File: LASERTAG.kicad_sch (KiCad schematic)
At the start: 38 parts, among them J1 Conn_01x02_Pin, J2 USB_C_Receptacle_USB2.0_14P, J3 Conn_01x02_Pin, SW1 SW_Push, SW2 SW_Push, SW3 SW_SPST, SW4 SW_SPST, U1 ATMEGA328-AU, U2 ESP32-S2-SOLO, U3 TPS613221ADBVR, U4 TPS613221ADBVR, U5 AP7366-33W5-7, U6 TSOP582xx, U7 TLV61048DBVR

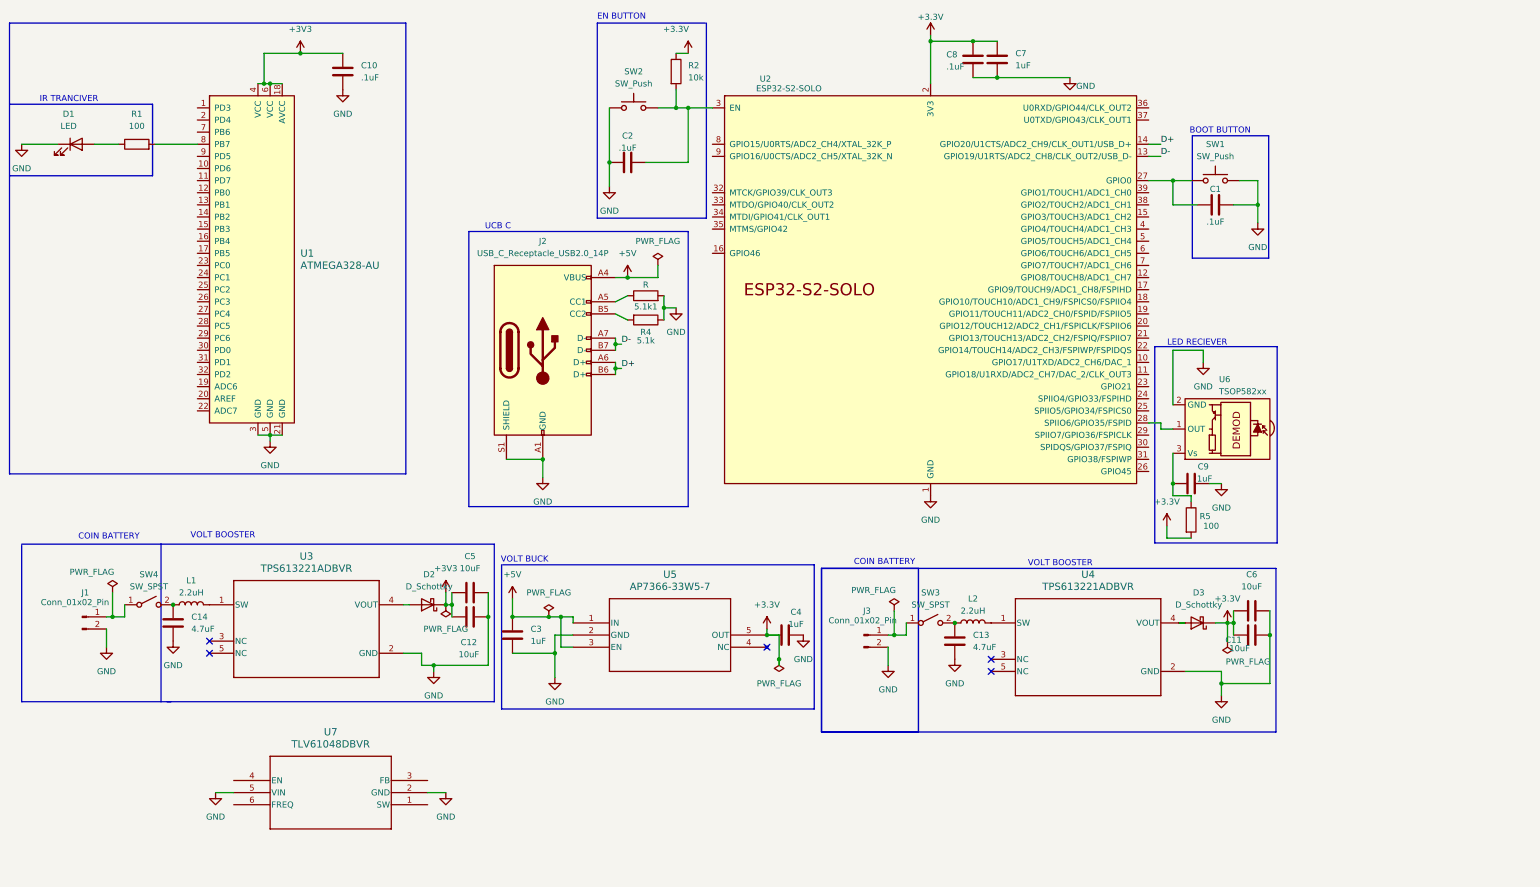
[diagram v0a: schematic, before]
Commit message: fix a lot of things i don't remember sorryy
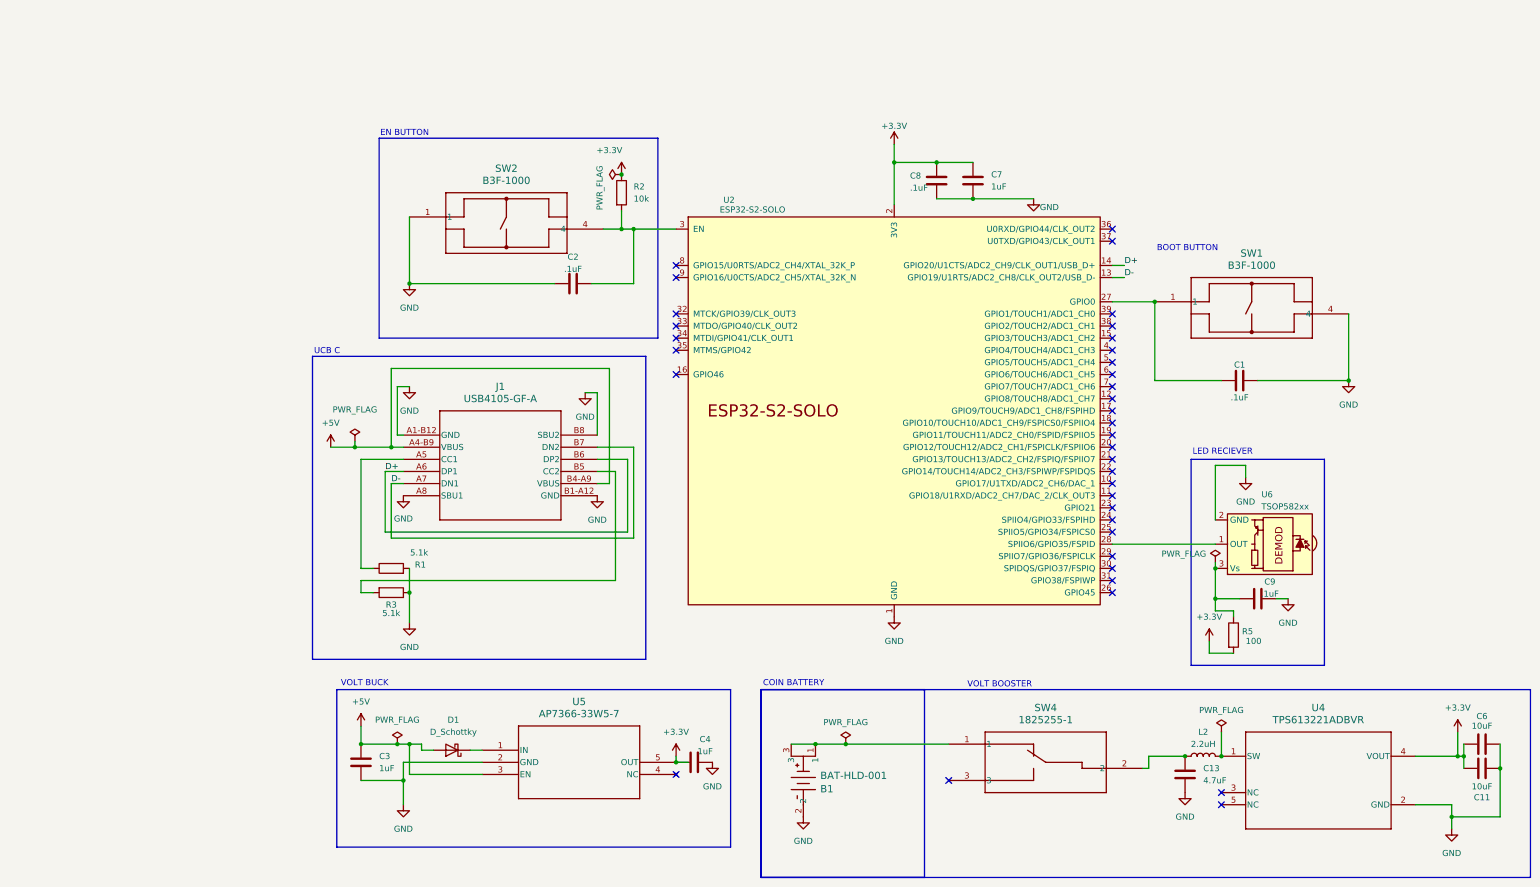
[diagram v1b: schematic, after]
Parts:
- removed 5.1k1: R, Resistor_SMD:R_0805_2012Metric, symbol Device:R
- removed C10: .1uF, Capacitor_SMD:C_0805_2012Metric, symbol Device:C
- removed C12, C5: 10uF, Capacitor_SMD:C_0805_2012Metric, symbol Device:C
- removed C14: 4.7uF, Capacitor_SMD:C_0805_2012Metric, symbol Device:C
- removed D1: LED, LED_SMD:LED_0805_2012Metric, symbol Device:LED
- removed D2, D3: D_Schottky, Diode_SMD:D_3220_8050Metric, symbol Device:D_Schottky
- removed J1, J3: Conn_01x02_Pin, symbol Connector:Conn_01x02_Pin
- removed J2: USB_C_Receptacle_USB2.0_14P, symbol Connector:USB_C_Receptacle_USB2.0_14P
- removed L1: 2.2uH, Inductor_SMD:L_0805_2012Metric, symbol Device:L
- removed R4: 5.1k, Resistor_SMD:R_0805_2012Metric, symbol Device:R
- removed SW1, SW2: SW_Push, symbol Switch:SW_Push
- removed SW3, SW4: SW_SPST, symbol Switch:SW_SPST
- removed U1: ATMEGA328-AU, digikey-footprints:TQFP-32_7x7mm, symbol dk_Embedded-Microcontrollers:ATMEGA328-AU
- removed U3: TPS613221ADBVR, DBV0005A_N, symbol 2024-10-19_05-20-17:TPS613221ADBVR
- removed U7: TLV61048DBVR, footprints:SOT-23-6_DBV_TEX, symbol 2024-11-02_21-57-25:TLV61048DBVR
- added B1: BAT-HLD-001, BAT_HLD_001:BATT_HLDR_LNX, symbol 2024-11-03_05-52-53:BAT-HLD-001
- added D1: D_Schottky, Diode_SMD:D_3220_8050Metric, symbol Device:D_Schottky
- added J1: USB4105-GF-A, USB4105_GF_A_2:GCT_USB4105-GF-A, symbol 2024-11-03_05-17-58:USB4105-GF-A
- added R3: 5.1k, Resistor_SMD:R_0805_2012Metric, symbol Device:R
- added SW1, SW2: B3F-1000, B3F_1000:SW_B3F-1000_OMR, symbol 2024-11-03_04-49-53:B3F-1000
- added SW4: 1825255-1, 1825255_1:SW3_1825255-1_TEC, symbol 2024-11-03_03-58-19:1825255-1
- R1: value 100 -> 5.1k
- U2: footprint PCM_Espressif:ESP32-S2-SOLO -> ESP32_S2_SOLO_N4:XCVR_ESP32-S2-SOLO-N4
- U4: footprint DBV0005A_N -> TPS613221ADBVR:DBV0005A_N
- U5: footprint SOT25-YE_DIO -> AP7366_33W5_7:SOT25-YE_DIO
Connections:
- net +3.3V: now also U4.4 (VOUT)
- net +5V: now also D1.2 (A), J1.A4-B9 (VBUS), J1.B4-A9 (VBUS); no longer U5.1 (IN)
- net D+: now also J1.A6 (DP1), J1.B6 (DP2)
- net D-: now also J1.A7 (DN1), J1.B7 (DN2)
- net GND: now also R1.2, B1.2, J1.A1-B12 (GND), J1.A8 (SBU1), J1.B1-A12 (GND), J1.B8 (SBU2), R3.1, SW1.4, SW2.1
- net at C2.2, R2.2, U2.3 (EN): now also SW2.4
- net at C13.1, L2.1: now also SW4.2
- net at C1.1, U2.27 (GPIO0): now also SW1.1
- net at R1.1: now also J1.A5 (CC1)
- new net: D1.1 (K), U5.1 (IN)
- new net: J1.B5 (CC2), R3.2
- new net: B1.1, B1.3, SW4.1
- no-connect marks 5 -> 36
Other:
- note removed: "IR TRANCIVER"
- moved on the sheet: C11, C13, C2, C3, C4, C6, C7, C8, C9, L2, R2, R5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
